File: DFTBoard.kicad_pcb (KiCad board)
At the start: 8 copper layers, 148.5 x 62 mm, 86 parts, among them CON1 AVR-JTAG-10, CON2 AVR-JTAG-10, J1 AUDIO JACK, J2 JACK_TRS_4PINS, J3 AUDIO JACK, J4 AUDIO JACK, J5 Micro_SD_Card_Det, J6 USB_A, J7 USB_B, SW1 TL6215RF200BDT, U10 VL53L0X, U11 APDS-9960, U12 MT41K256M16HA-125_E, U13 MT41K256M16HA-125_E, U5 xc7z020clg400, U6 TLV320AIC3104, U9 MIC2025-1YMM, Y1 Crystal, Y2 Crystal

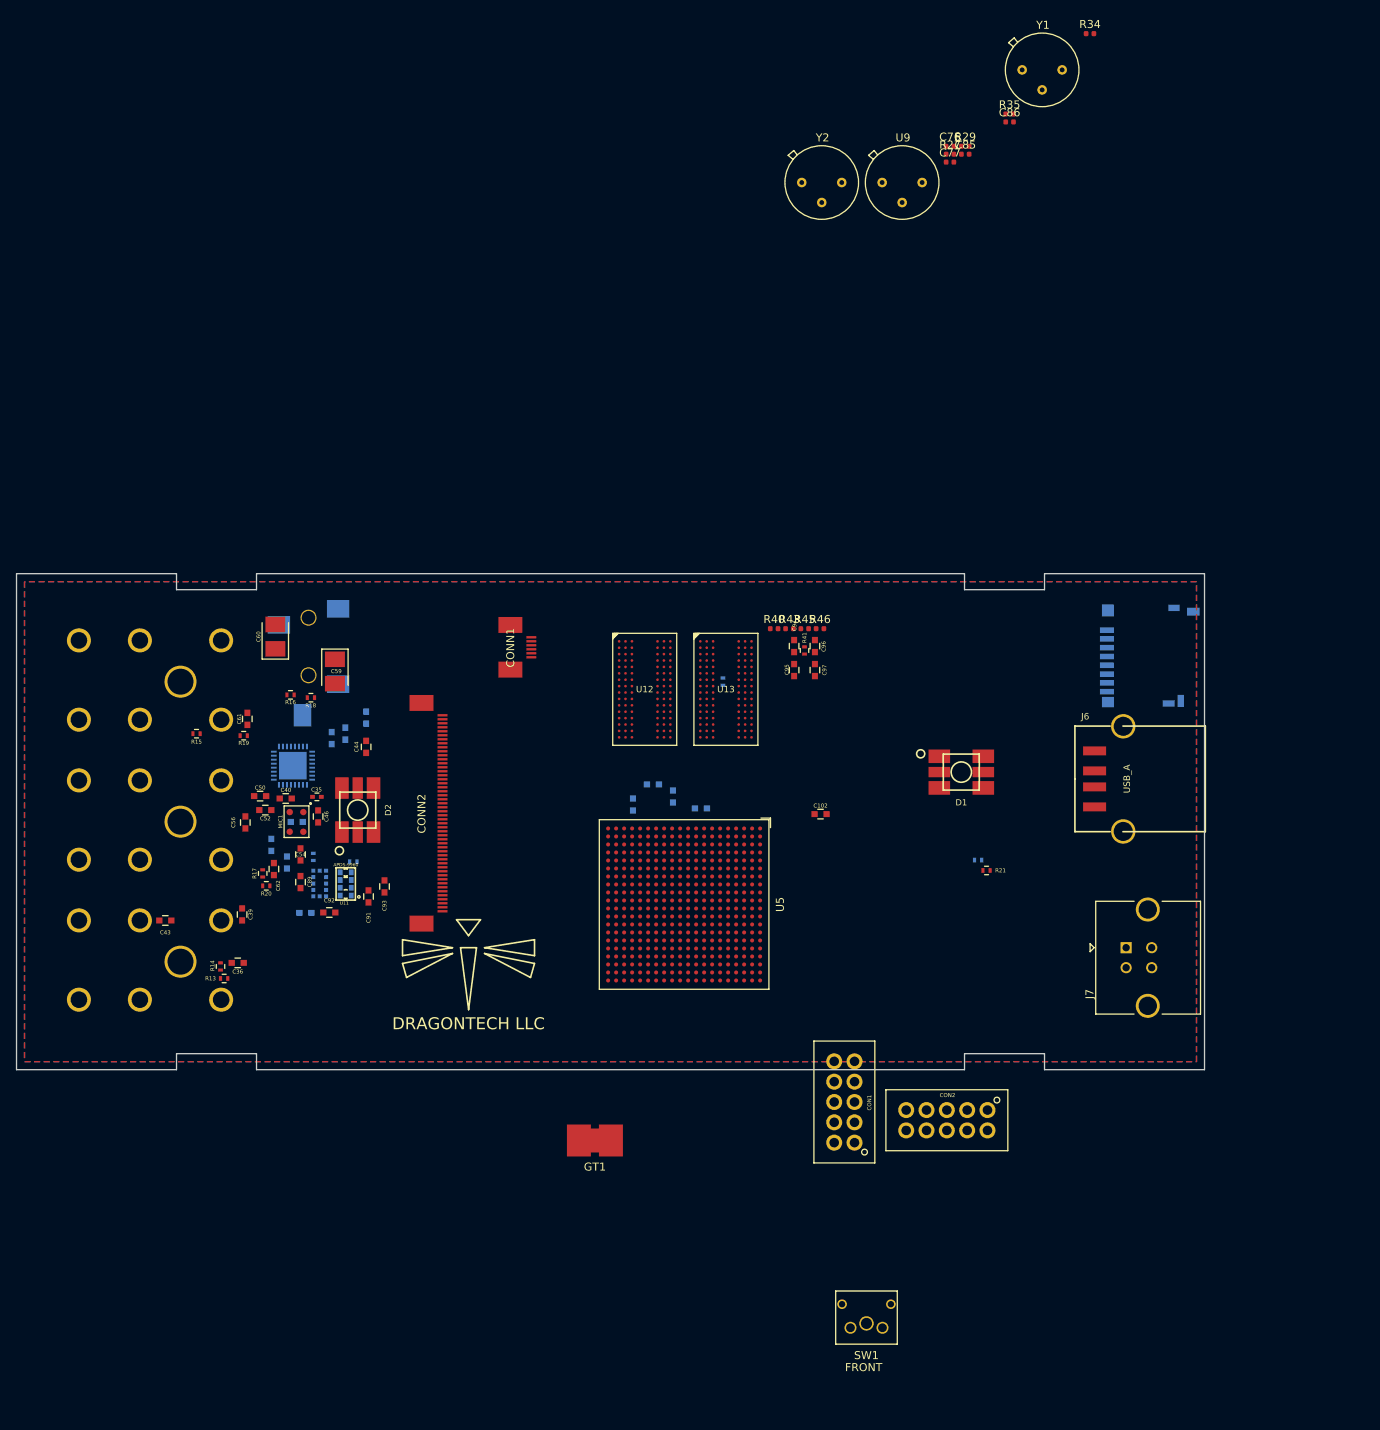
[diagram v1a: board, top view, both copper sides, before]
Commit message: random updates
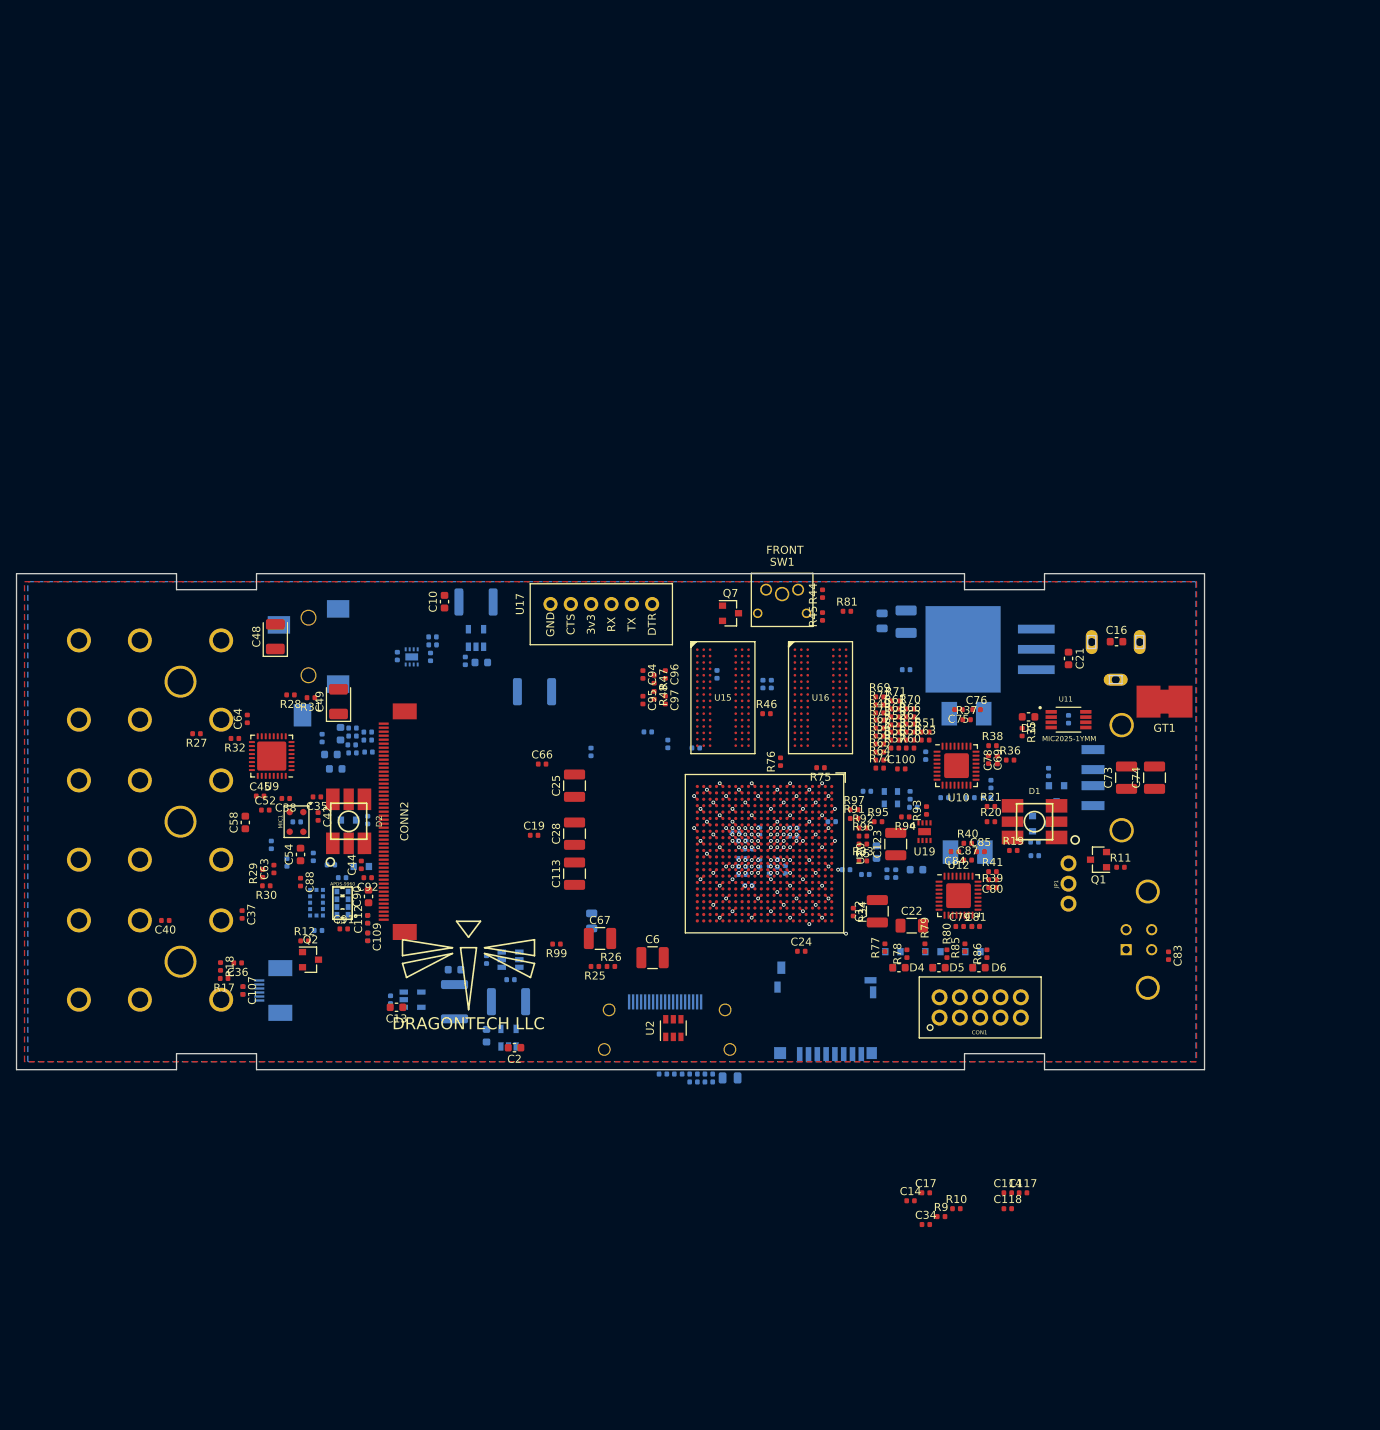
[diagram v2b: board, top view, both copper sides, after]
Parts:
- removed CON2: AVR-JTAG-10, DFTcustom:XilinxJTAG
- removed the J5 at (247.8, 103.2)
- removed the R37 at (143.6, 128.4)
- removed the R40 at (201.2, 99.9)
- removed the R41 at (205.0, 102.6)
- removed the U13 at (195.2, 107.5)
- added C1: .47uF, Capacitor_SMD:C_0402_1005Metric, B.Cu at (165.2, 141.2)
- added C10: 10uF, Capacitor_SMD:C_0603_1608Metric, F.Cu at (160.0, 96.5)
- added C100: 4.7uF, Capacitor_SMD:C_0402_1005Metric, F.Cu at (217.1, 117.4)
- added C101: .47uF, Capacitor_SMD:C_0402_1005Metric, B.Cu at (185.4, 112.8)
- added C103: .47uF, Capacitor_SMD:C_0402_1005Metric, B.Cu at (191.4, 114.8)
- added C108: 4.7uF, Capacitor_SMD:C_0402_1005Metric, B.Cu at (134.8, 145.1)
- added C109: .1uF, Capacitor_SMD:C_0402_1005Metric, F.Cu at (150.4, 138.4)
- added C11: 10uF, Capacitor_SMD:C_0603_1608Metric, B.Cu at (165.2, 150.8)
- added C110: 4.7uF, Capacitor_SMD:C_0402_1005Metric, B.Cu at (150.4, 138.4)
- added C111: .1uF, Capacitor_SMD:C_0402_1005Metric, B.Cu at (150.4, 136.2)
- added C112: 4.7uF, Capacitor_SMD:C_0402_1005Metric, F.Cu at (150.4, 136.2)
- added C113: 47uF, Capacitor_SMD:C_1210_3225Metric, F.Cu at (176.2, 130.5)
- added C114: 4.7uF, Capacitor_SMD:C_0402_1005Metric, F.Cu at (230.4, 170.4)
- added C115: 4.7uF, Capacitor_SMD:C_0402_1005Metric, B.Cu at (216.4, 130.5)
- added C116: .47uF, Capacitor_SMD:C_0402_1005Metric, B.Cu at (198.0, 127.4)
- added C117: .47uF, Capacitor_SMD:C_0402_1005Metric, F.Cu at (232.3, 170.4)
- added C118: .47uF, Capacitor_SMD:C_0402_1005Metric, F.Cu at (230.4, 172.4)
- added C119: .47uF, Capacitor_SMD:C_0402_1005Metric, B.Cu at (199.4, 125.2)
- added C12: 100uF, Capacitor_SMD:C_1210_3225Metric, F.Cu at (214.1, 135.2)
- added C120: .01uF, Capacitor_SMD:C_0402_1005Metric, B.Cu at (218.2, 120.7)
- added C121: .47uF, Capacitor_SMD:C_0402_1005Metric, B.Cu at (210.2, 130.0)
- added C122: 4.7uF, Capacitor_SMD:C_0402_1005Metric, B.Cu at (208.4, 124.0)
- added C123: 100uF, Capacitor_SMD:C_1210_3225Metric, F.Cu at (216.4, 126.8)
- added C13: 10uF, Capacitor_SMD:C_0603_1608Metric, F.Cu at (154.0, 147.2)
- added C14: .47uF, Capacitor_SMD:C_0402_1005Metric, F.Cu at (218.3, 171.4)
- added C15: .47uF, Capacitor_SMD:C_0402_1005Metric, B.Cu at (202.6, 130.0)
- added C16: 10uF, Capacitor_SMD:C_0603_1608Metric, F.Cu at (244.0, 101.5)
- added C17: .47uF, Capacitor_SMD:C_0402_1005Metric, F.Cu at (220.2, 170.4)
- added C18: .47uF, Capacitor_SMD:C_0402_1005Metric, B.Cu at (197.2, 129.6)
- added C19: 4.7uF, Capacitor_SMD:C_0402_1005Metric, F.Cu at (171.2, 125.7)
- added C2: 10uF, Capacitor_SMD:C_0603_1608Metric, F.Cu at (168.8, 152.2)
- added C20: 4.7uF, Capacitor_SMD:C_0402_1005Metric, B.Cu at (201.6, 129.2)
- added C21: 10uF, Capacitor_SMD:C_0603_1608Metric, F.Cu at (238.0, 103.6)
- added C22: 330uF, Capacitor_SMD:C_1206_3216Metric, F.Cu at (218.4, 137.0)
- added C23: .47uF, Capacitor_SMD:C_0402_1005Metric, B.Cu at (197.2, 126.4)
- added C24: 4.7uF, Capacitor_SMD:C_0402_1005Metric, F.Cu at (204.6, 140.2)
- added C25: 100uF, Capacitor_SMD:C_1210_3225Metric, F.Cu at (176.2, 119.5)
- added C26: 10uF, Capacitor_SMD:C_0603_1608Metric, B.Cu at (161.2, 142.5)
- added C27: 4.7uF, Capacitor_SMD:C_0402_1005Metric, B.Cu at (215.3, 130.5)
- added C28: 100uF, Capacitor_SMD:C_1210_3225Metric, F.Cu at (176.2, 125.5)
- added C29: .47uF, Capacitor_SMD:C_0402_1005Metric, B.Cu at (203.6, 125.8)
- added C3: 10uF, Capacitor_SMD:C_0603_1608Metric, B.Cu at (164.6, 104.1)
- added C30: .47uF, Capacitor_SMD:C_0402_1005Metric, B.Cu at (203.6, 124.8)
- added C31: .47uF, Capacitor_SMD:C_0402_1005Metric, B.Cu at (197.2, 130.6)
- added C32: 47uF, Capacitor_SMD:C_0805_2012Metric, B.Cu at (178.4, 136.4)
- added C33: 10uF, Capacitor_SMD:C_0603_1608Metric, B.Cu at (214.0, 127.8)
- added C34: .47uF, Capacitor_SMD:C_0402_1005Metric, F.Cu at (220.2, 174.4)
- added C37: 1uF, Capacitor_SMD:C_0402_1005Metric, F.Cu at (134.7, 135.6)
- added C38: 1uF, Capacitor_SMD:C_0402_1005Metric, F.Cu at (140.2, 121.1)
- added C4: .47uF, Capacitor_SMD:C_0402_1005Metric, B.Cu at (196.4, 125.4)
- added C42: 4.7uF, Capacitor_SMD:C_0402_1005Metric, F.Cu at (144.2, 123.3)
- added C45: 1uF, Capacitor_SMD:C_0402_1005Metric, F.Cu at (136.9, 120.8)
- added C47: .47uF, Capacitor_SMD:C_0402_1005Metric, B.Cu at (191.1, 155.5)
- added C48: 220uF Tant., Capacitor_Tantalum_SMD:CP_EIA-3528-12_Kemet-T, F.Cu at (138.8, 100.9)
- added C49: 220uF Tant., Capacitor_Tantalum_SMD:CP_EIA-3528-12_Kemet-T, F.Cu at (146.8, 109.0)
- added C5: 4.7uF, Capacitor_SMD:C_0402_1005Metric, B.Cu at (197.2, 128.6)
- added C6: 100uF, Capacitor_SMD:C_1210_3225Metric, F.Cu at (186.0, 141.0)
- added C63: .1uF, Capacitor_SMD:C_0402_1005Metric, F.Cu at (138.7, 129.9)
- added C64: .1uF, Capacitor_SMD:C_0402_1005Metric, F.Cu at (135.3, 111.2)
- added C65: .47uF, Capacitor_SMD:C_0402_1005Metric, B.Cu at (198.0, 132.0)
- added C66: 4.7uF, Capacitor_SMD:C_0402_1005Metric, F.Cu at (172.2, 116.8)
- added C67: 100uF, Capacitor_SMD:C_1210_3225Metric, F.Cu at (179.4, 138.6)
- added C68: .1uF, Capacitor_SMD:C_0402_1005Metric, B.Cu at (225.8, 121.0)
- added C69: 2.2uF, Capacitor_SMD:C_0402_1005Metric, F.Cu at (228.0, 116.2)
- added C7: 47uF, Capacitor_SMD:C_0805_2012Metric, B.Cu at (214.7, 98.9)
- added C70: .1uF, Capacitor_SMD:C_0402_1005Metric, B.Cu at (220.2, 115.8)
- added C71: .1uF, Capacitor_SMD:C_0402_1005Metric, B.Cu at (222.5, 121.0)
- added C72: .1uF, Capacitor_SMD:C_0402_1005Metric, B.Cu at (238.0, 111.2)
- added C73: 100uF, Capacitor_SMD:C_1210_3225Metric, F.Cu at (245.2, 118.5)
- added C74: 100uF, Capacitor_SMD:C_1210_3225Metric, F.Cu at (248.8, 118.5)
- added C77: .1uF, Capacitor_SMD:C_0402_1005Metric, B.Cu at (227.8, 121.0)
- added C78: .47uF, Capacitor_SMD:C_0402_1005Metric, F.Cu at (229.1, 116.3)
- added C79: .1uF, Capacitor_SMD:C_0402_1005Metric, F.Cu at (224.4, 137.1)
- added C8: .47uF, Capacitor_SMD:C_0402_1005Metric, B.Cu at (199.4, 129.2)
- added C80: 2.2uF, Capacitor_SMD:C_0402_1005Metric, F.Cu at (228.5, 131.2)
- added C81: .1uF, Capacitor_SMD:C_0402_1005Metric, F.Cu at (226.4, 137.1)
- added C82: .1uF, Capacitor_SMD:C_0402_1005Metric, B.Cu at (226.4, 137.1)
- added C83: 4.7uF, Capacitor_SMD:C_0402_1005Metric, F.Cu at (250.5, 140.8)
- added C86: .1uF, Capacitor_SMD:C_0402_1005Metric, B.Cu at (228.3, 119.3)
- added C87: .47uF, Capacitor_SMD:C_0402_1005Metric, F.Cu at (225.4, 128.8)
- added C88: .1uF, Capacitor_SMD:C_0402_1005Metric, F.Cu at (142.0, 131.6)
- added C9: 4.7uF, Capacitor_SMD:C_0402_1005Metric, B.Cu at (200.6, 130.0)
- added C98: .01uF, Capacitor_SMD:C_0402_1005Metric, B.Cu at (217.7, 105.0)
- added C99: 100uF, Capacitor_SMD:C_1210_3225Metric, B.Cu at (217.7, 99.0)
- added D3: BLUE LED, Capacitor_SMD:C_0603_1608Metric, F.Cu at (233.0, 110.9)
- added D4: BLUE LED, Capacitor_SMD:C_0603_1608Metric, F.Cu at (216.8, 142.2)
- added D5: BLUE LED, Capacitor_SMD:C_0603_1608Metric, F.Cu at (221.8, 142.2)
- added D6: BLUE LED, Capacitor_SMD:C_0603_1608Metric, F.Cu at (226.8, 142.2)
- added FB1: 120Ω @ 100 MHz, size 0603, Capacitor_SMD:C_0603_1608Metric, B.Cu at (219.0, 130.0)
- added J1: PJ-102A, PJ-102A:CUI_PJ-102A, B.Cu at (247.4, 101.5)
- added J8: Micro_SD_Card_Det, DFTcustom:AMPHENOL-114-00841-68, B.Cu at (207.6, 148.0)
- added J9: HDMI_A, DFTcustom:10029449-111RLF, B.Cu at (187.8, 152.5)
- added JP1: Jumper_3_Open, DFTcustom:JUMPER_3PIN, F.Cu at (238.0, 131.8)
- added L1: 2.2uH, Capacitor_SMD:C_1812_4532Metric, B.Cu at (171.2, 107.8)
- added L2: 2.2uH, Capacitor_SMD:C_1812_4532Metric, B.Cu at (163.9, 96.5)
- added L3: 2.2uH, Capacitor_SMD:C_1812_4532Metric, B.Cu at (168.0, 146.5)
- added L4: 2.2uH, Capacitor_SMD:C_1812_4532Metric, B.Cu at (161.2, 146.5)
- added Q1: IRLML2502, Package_TO_SOT_SMD:SOT-23, F.Cu at (241.8, 128.8)
- added Q10: IRLML2502, Package_TO_SOT_SMD:SOT-23, B.Cu at (226.1, 141.2)
- added Q2: IRLML2502, Package_TO_SOT_SMD:SOT-23, F.Cu at (143.2, 141.2)
- added Q3: IRLML2502, Package_TO_SOT_SMD:SOT-23, B.Cu at (234.5, 124.2)
- added Q4: IRLML2502, Package_TO_SOT_SMD:SOT-23, B.Cu at (148.0, 124.8)
- added Q5: IRLML2502, Package_TO_SOT_SMD:SOT-23, B.Cu at (236.5, 120.5)
- added Q6: IRLML2502, Package_TO_SOT_SMD:SOT-23, B.Cu at (149.6, 128.6)
- added Q7: IRLML2502, Package_TO_SOT_SMD:SOT-23, F.Cu at (195.8, 98.0)
- added Q8: IRLML2502, Package_TO_SOT_SMD:SOT-23, B.Cu at (216.1, 141.2)
- added Q9: IRLML2502, Package_TO_SOT_SMD:SOT-23, B.Cu at (221.1, 141.2)
- added R1: 100k, Resistor_SMD:R_0402_1005Metric, B.Cu at (168.2, 143.8)
- added R10: 4.7k, Resistor_SMD:R_0402_1005Metric, F.Cu at (224.0, 172.4)
- added R100: 24.9 1%, Resistor_SMD:R_0402_1005Metric, B.Cu at (212.8, 120.2)
- added R11: 100, Resistor_SMD:R_0402_1005Metric, F.Cu at (244.5, 129.7)
- added R12: 100, Resistor_SMD:R_0402_1005Metric, F.Cu at (142.5, 138.9)
- added R2: 100k, Resistor_SMD:R_0402_1005Metric, B.Cu at (153.2, 146.2)
- added R23: 100, Resistor_SMD:R_0402_1005Metric, B.Cu at (148.0, 121.5)
- added R24: 150, Resistor_SMD:R_0402_1005Metric, B.Cu at (150.0, 121.5)
- added R25: 4.7k, Resistor_SMD:R_0402_1005Metric, F.Cu at (178.8, 142.1)
- added R26: 4.7k, Resistor_SMD:R_0402_1005Metric, F.Cu at (180.8, 142.1)
- added R27: 100k, Resistor_SMD:R_0402_1005Metric, F.Cu at (129.0, 113.0)
- added R28: 100k, Resistor_SMD:R_0402_1005Metric, F.Cu at (140.8, 108.2)
- added R29: 100k, Resistor_SMD:R_0402_1005Metric, F.Cu at (137.3, 130.5)
- added R3: 100k, Resistor_SMD:R_0402_1005Metric, B.Cu at (162.6, 103.9)
- added R30: 49.9k, Resistor_SMD:R_0402_1005Metric, F.Cu at (137.7, 132.0)
- added R31: 49.9k, Resistor_SMD:R_0402_1005Metric, F.Cu at (143.3, 108.5)
- added R32: 49.9k, Resistor_SMD:R_0402_1005Metric, F.Cu at (133.8, 113.6)
- added R33: 10k, Resistor_SMD:R_0402_1005Metric, F.Cu at (212.3, 128.9)
- added R34: 47, Resistor_SMD:R_0402_1005Metric, F.Cu at (211.1, 135.3)
- added R35: 150, Resistor_SMD:R_0402_1005Metric, F.Cu at (232.2, 112.8)
- added R39: 10k, Resistor_SMD:R_0402_1005Metric, F.Cu at (228.5, 132.2)
- added R4: 100k, Resistor_SMD:R_0402_1005Metric, B.Cu at (154.1, 103.3)
- added R42: 10k, Resistor_SMD:R_0402_1005Metric, B.Cu at (145.8, 129.4)
- added R47: 10k 1%, Resistor_SMD:R_0402_1005Metric, F.Cu at (186.2, 106.2)
- added R48: 10k 1%, Resistor_SMD:R_0402_1005Metric, F.Cu at (186.2, 108.2)
- added R49: 240 1%, Resistor_SMD:R_0402_1005Metric, F.Cu at (214.4, 110.4)
- added R5: 100k, Resistor_SMD:R_0402_1005Metric, F.Cu at (212.3, 126.8)
- added R50: 100, Resistor_SMD:R_0402_1005Metric, B.Cu at (194.1, 105.6)
- added R51: 40.2 1%, Resistor_SMD:R_0402_1005Metric, F.Cu at (220.1, 112.8)
- added R52: 40.2 1%, Resistor_SMD:R_0402_1005Metric, F.Cu at (216.3, 111.9)
- added R53: 40.2 1%, Resistor_SMD:R_0402_1005Metric, F.Cu at (216.3, 112.8)
- added R54: 40.2 1%, Resistor_SMD:R_0402_1005Metric, F.Cu at (214.4, 113.3)
- added R55: 40.2 1%, Resistor_SMD:R_0402_1005Metric, F.Cu at (218.2, 112.8)
- added R56: 40.2 1%, Resistor_SMD:R_0402_1005Metric, F.Cu at (216.3, 113.8)
- added R57: 40.2 1%, Resistor_SMD:R_0402_1005Metric, F.Cu at (216.3, 114.8)
- added R58: 40.2 1%, Resistor_SMD:R_0402_1005Metric, F.Cu at (218.2, 113.8)
- added R59: 40.2 1%, Resistor_SMD:R_0402_1005Metric, F.Cu at (214.4, 114.3)
- added R6: 10k, Resistor_SMD:R_0402_1005Metric, B.Cu at (158.2, 103.4)
- added R60: 40.2 1%, Resistor_SMD:R_0402_1005Metric, F.Cu at (218.2, 114.8)
- added R61: 40.2 1%, Resistor_SMD:R_0402_1005Metric, F.Cu at (216.3, 109.9)
- added R62: 40.2 1%, Resistor_SMD:R_0402_1005Metric, F.Cu at (218.2, 111.8)
- added R63: 40.2 1%, Resistor_SMD:R_0402_1005Metric, F.Cu at (220.1, 113.8)
- added R64: 40.2 1%, Resistor_SMD:R_0402_1005Metric, F.Cu at (214.4, 116.3)
- added R65: 40.2 1%, Resistor_SMD:R_0402_1005Metric, F.Cu at (214.4, 115.3)
- added R66: 40.2 1%, Resistor_SMD:R_0402_1005Metric, F.Cu at (218.2, 110.9)
- added R67: 40.2 1%, Resistor_SMD:R_0402_1005Metric, F.Cu at (214.4, 112.3)
- added R68: 40.2 1%, Resistor_SMD:R_0402_1005Metric, F.Cu at (216.3, 110.9)
- added R69: 40.2 1%, Resistor_SMD:R_0402_1005Metric, F.Cu at (214.4, 108.4)
- added R7: 240 1%, Resistor_SMD:R_0402_1005Metric, B.Cu at (158.5, 101.9)
- added R70: 40.2 1%, Resistor_SMD:R_0402_1005Metric, F.Cu at (218.2, 109.9)
- added R71: 40.2 1%, Resistor_SMD:R_0402_1005Metric, F.Cu at (216.4, 108.9)
- added R72: 40.2 1%, Resistor_SMD:R_0402_1005Metric, F.Cu at (214.4, 109.4)
- added R73: 40.2 1%, Resistor_SMD:R_0402_1005Metric, F.Cu at (214.4, 111.3)
- added R74: 4.7k, Resistor_SMD:R_0402_1005Metric, F.Cu at (214.4, 117.3)
- added R75: 80.6, Resistor_SMD:R_0402_1005Metric, F.Cu at (207.0, 117.2)
- added R76: 80.6, Resistor_SMD:R_0402_1005Metric, F.Cu at (202.0, 116.5)
- added R77: 1k, Resistor_SMD:R_0402_1005Metric, F.Cu at (215.1, 139.8)
- added R78: 150, Resistor_SMD:R_0402_1005Metric, F.Cu at (217.8, 140.5)
- added R79: 1k, Resistor_SMD:R_0402_1005Metric, F.Cu at (220.1, 139.8)
- added R8: 4.7k, Resistor_SMD:R_0402_1005Metric, B.Cu at (158.5, 100.9)
- added R80: 150, Resistor_SMD:R_0402_1005Metric, F.Cu at (222.8, 140.5)
- added R81: 10k, Resistor_SMD:R_0402_1005Metric, F.Cu at (210.3, 97.7)
- added R82: 10k, Resistor_SMD:R_0402_1005Metric, B.Cu at (150.5, 115.3)
- added R83: 10k, Resistor_SMD:R_0402_1005Metric, B.Cu at (148.5, 115.4)
- added R84: 10k, Resistor_SMD:R_0402_1005Metric, B.Cu at (148.4, 114.4)
- added R85: 1k, Resistor_SMD:R_0402_1005Metric, F.Cu at (225.1, 139.8)
- added R86: 150, Resistor_SMD:R_0402_1005Metric, F.Cu at (227.8, 140.5)
- added R87: 33, Resistor_SMD:R_0402_1005Metric, B.Cu at (150.4, 113.8)
- added R88: 33, Resistor_SMD:R_0402_1005Metric, B.Cu at (148.5, 113.3)
- added R89: 33, Resistor_SMD:R_0402_1005Metric, B.Cu at (150.4, 112.8)
- added R9: 4.7k, Resistor_SMD:R_0402_1005Metric, F.Cu at (222.1, 173.4)
- added R90: 33, Resistor_SMD:R_0402_1005Metric, B.Cu at (148.5, 112.3)
- added R91: 20k, Resistor_SMD:R_0402_1005Metric, F.Cu at (211.2, 123.6)
- added R92: 20k, Resistor_SMD:R_0402_1005Metric, F.Cu at (212.3, 124.8)
- added R93: 20k, Resistor_SMD:R_0402_1005Metric, F.Cu at (220.2, 122.6)
- added R94: 20k, Resistor_SMD:R_0402_1005Metric, F.Cu at (217.6, 123.4)
- added R95: 20k, Resistor_SMD:R_0402_1005Metric, F.Cu at (214.2, 124.0)
- added R96: 20k, Resistor_SMD:R_0402_1005Metric, F.Cu at (212.3, 125.8)
- added R97: 20k, Resistor_SMD:R_0402_1005Metric, F.Cu at (211.2, 122.5)
- added R98: 4.7k, Resistor_SMD:R_0402_1005Metric, B.Cu at (218.6, 122.2)
- added R99: 47k, Resistor_SMD:R_0402_1005Metric, F.Cu at (174.0, 139.3)
- added U1: LM3880, Package_TO_SOT_SMD:SOT-23-6, B.Cu at (168.2, 141.2)
- added U10: USB3320, Package_DFN_QFN:QFN-32-1EP_5x5mm_P0.5mm_EP3.1x3.1mm, F.Cu at (224.0, 117.0)
- added U11: MIC2025-1YMM, SOP65P490X110-8N:SOP65P490X110-8N, F.Cu at (238.0, 111.2)
- added U12: USB3320, Package_DFN_QFN:QFN-32-1EP_5x5mm_P0.5mm_EP3.1x3.1mm, F.Cu at (224.2, 133.2)
- added U16: MT41K256M16HA-125_E, DFTcustom:FBGA-96-DDR3-SDRAM, F.Cu at (207.0, 108.5)
- added U17: FTDITypeUART, DFTcustom:FTDI_CONN, F.Cu at (179.6, 96.8)
- added U18: ABRACON-ASDMB, XTAL_ASDMB-24.000MHZ-LC-T:XTAL_ASDMB-24.000MHZ-LC-T, B.Cu at (215.8, 121.0)
- added U19: S25FL256SAGNFI001, DFTcustom:WSON-8, F.Cu at (220.0, 125.2)
- added U2: LM3880, Package_TO_SOT_SMD:SOT-23-6, F.Cu at (188.6, 149.8)
- added U20: xc7z020clg484, DFTcustom:BGA-484_19.0x19.0mm_Layout22x22_P0.80mm_dia0.40mm, F.Cu at (200.0, 128.0)
- added U3: SC189 - 1.0V, Package_TO_SOT_SMD:SOT-23-5, B.Cu at (168.0, 151.0)
- added U4: SC189 - 3.3V, Package_TO_SOT_SMD:SOT-23-5, B.Cu at (163.9, 101.0)
- added U7: SC189 - 1.8V, Package_TO_SOT_SMD:SOT-23-5, B.Cu at (156.0, 146.2)
- C102, C46: value 4.7uF -> .47uF; footprint Capacitors_SMD:C_0603 -> Capacitor_SMD:C_0402_1005Metric; moved to B.Cu
- C104, C36, C40, C52, C53, C92, C94, C95, C96, C97: footprint Capacitors_SMD:C_0603 -> Capacitor_SMD:C_0402_1005Metric
- C105, C106: value .47uF -> .01uF; footprint Capacitors_SMD:C_0603 -> Capacitor_SMD:C_0402_1005Metric
- C107: value .47uF -> .1uF; footprint Capacitors_SMD:C_0603 -> Capacitor_SMD:C_0402_1005Metric; moved to F.Cu
- C35: footprint Capacitors_SMD:C_0402 -> Capacitor_SMD:C_0402_1005Metric
- C39: value 1uF -> .1uF; footprint Capacitors_SMD:C_0603 -> Capacitor_SMD:C_0402_1005Metric; moved to B.Cu
- C41: value .1uF -> 10uF; footprint Capacitors_SMD:C_0603 -> Capacitor_SMD:C_0603_1608Metric
- C43, C62: footprint Capacitors_SMD:C_0603 -> Capacitor_SMD:C_0402_1005Metric; moved to B.Cu
- C44, C91: value 10uF -> 1uF; footprint Capacitors_SMD:C_0603 -> Capacitor_SMD:C_0402_1005Metric
- C50: value 1uF -> .47uF; footprint Capacitors_SMD:C_0603 -> Capacitor_SMD:C_0402_1005Metric; moved to B.Cu
- C51, C54: footprint Capacitors_SMD:C_0603 -> Capacitor_SMD:C_0603_1608Metric
- C55: value .1uF -> .47uF; footprint Capacitors_SMD:C_0603 -> Capacitor_SMD:C_0402_1005Metric
- C56: value 10uF -> .1uF; footprint Capacitors_SMD:C_0603 -> Capacitor_SMD:C_0402_1005Metric; moved to B.Cu
- C57: value 10uF -> 4.7uF; footprint Capacitors_SMD:C_0603 -> Capacitor_SMD:C_0402_1005Metric
- C58: value .1uF -> 10uF; footprint Capacitors_SMD:C_0603 -> Capacitor_SMD:C_0603_1608Metric; moved to F.Cu
- C59: value 220uF Tant. -> 4.7uF; footprint Capacitors_Tantalum_SMD:CP_Tantalum_Case-T_EIA-3528-12_Reflow -> Capacitor_SMD:C_0402_1005Metric; moved to B.Cu
- C60: value 220uF Tant. -> 10uF; footprint Capacitors_Tantalum_SMD:CP_Tantalum_Case-T_EIA-3528-12_Reflow -> Capacitor_SMD:C_0603_1608Metric; moved to B.Cu
- C61: value .1uF -> 47uF; footprint Capacitors_SMD:C_0603 -> Capacitor_SMD:C_0805_2012Metric; moved to B.Cu
- C89: value .1uF -> 4.7uF; footprint Capacitors_SMD:C_0603 -> Capacitor_SMD:C_0402_1005Metric; moved to B.Cu
- C90: value 4.7uF -> 10uF; footprint Capacitors_SMD:C_0603 -> Capacitor_SMD:C_0603_1608Metric; moved to F.Cu
- C93: value 1uF -> .01uF; footprint Capacitors_SMD:C_0603 -> Capacitor_SMD:C_0402_1005Metric; moved to B.Cu
- CONN1, J6, J7: moved to B.Cu
- R13, R15, R16: value 100k -> 100; footprint Resistors_SMD:R_0402 -> Resistor_SMD:R_0402_1005Metric; moved to B.Cu
- R14: value 49.9k -> 100; footprint Resistors_SMD:R_0402 -> Resistor_SMD:R_0402_1005Metric; moved to B.Cu
- R17, R18: footprint Resistors_SMD:R_0402 -> Resistor_SMD:R_0402_1005Metric
- R19, R20: value 49.9k -> 100; footprint Resistors_SMD:R_0402 -> Resistor_SMD:R_0402_1005Metric
- R21: value 4.7k -> 150; footprint Resistors_SMD:R_0402 -> Resistor_SMD:R_0402_1005Metric
- R22: value 4.7k -> 100; footprint Resistors_SMD:R_0402 -> Resistor_SMD:R_0402_1005Metric
- R36: footprint Resistors_SMD:R_0402 -> Resistor_SMD:R_0402_1005Metric; moved to F.Cu
- R43: value 240 1% -> 10k; moved to B.Cu
- R44: value 100 -> 10k; footprint Resistors_SMD:R_0402 -> Resistor_SMD:R_0402_1005Metric; moved to F.Cu
- R45: value 80.6 -> 150
- R46: value 80.6 -> 240 1%
- U5: value xc7z020clg400 -> TLV62080DSGx; footprint Package_BGA:BGA-400_21.0x21.0mm_Layout20x20_P1.0mm -> Package_SON:WSON-8-1EP_2x2mm_P0.5mm_EP0.9x1.6mm; moved to B.Cu
- U6: value TLV320AIC3104 -> LM1085-5.0; footprint Housings_DFN_QFN:QFN-32-1EP_5x5mm_Pitch0.5mm -> Package_TO_SOT_SMD:TO-263-3_TabPin2
- U9: value MIC2025-1YMM -> TLV320AIC3104; footprint Crystal:Crystal_HC35-U -> Package_DFN_QFN:QFN-32-1EP_5x5mm_P0.5mm_EP3.65x3.65mm
- Y1, Y2: value Crystal -> ABM3-24.000MHZ-D2Y-T; footprint Crystal:Crystal_HC35-U -> ABM3-12.000MHZ-B2-T:XTAL500X320X130N; moved to B.Cu
- moved C43 109.0 mm to (233.8, 128.2), turned to 0 degrees
- moved R15 106.6 mm to (235.5, 117.8), turned to 90 degrees
- moved U9 104.7 mm to (138.4, 115.8), turned to 180 degrees
- moved R13 102.7 mm to (233.8, 126.5)
- moved R40 102.4 mm to (225.4, 126.7)
- moved R19 97.3 mm to (231.1, 127.6), turned to 0 degrees
- moved SW1 96.9 mm to (202.2, 93.0), turned to 180 degrees
- moved R41 94.7 mm to (228.5, 130.2)
- moved C85 91.3 mm to (227.0, 127.8)
- moved R20 90.9 mm to (228.3, 124.0), turned to 0 degrees
- moved GT1 89.9 mm to (250.0, 109.0)
- moved U6 88.4 mm to (228.2, 102.5)
- moved C84 87.2 mm to (223.8, 127.8), turned to 180 degrees
- moved Y2 86.2 mm to (225.4, 127.8)
- moved R36 83.1 mm to (230.7, 116.3), turned to 0 degrees
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- renumbered C76 to C75, C77 to C76, C85 to C84, C86 to C85, J1 to J2, J4 to J3, J3 to J4, J2 to J5, R27 to R37, R29 to R38, R34 to R40, R35 to R41, U10 to U13, U11 to U14, U12 to U15
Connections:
- C102 pad 1: Net-(C100-Pad1) -> +1V35
- C104 pad 1: Net-(C100-Pad1) -> +1V35
- C105 pad 1: Net-(C100-Pad1) -> /DDR3/VREF
- C106 pad 1: Net-(C100-Pad1) -> /DDR3/VREF
- C107 pad 1: Net-(C100-Pad1) -> +3V3
- C39 pad 1: /Audio/JACK_INC_P -> GND
- C39 pad 2: /Audio/JACK_IN_P -> +1V8
- C40 pad 1: /Audio/SIG_F -> /Audio/JACK_INC_N
- C40 pad 2: /Audio/SIGC_F -> /Audio/JACK_IN_N
- C41 pad 2: +1.8V -> +1V8
- C43 pad 1: /Audio/JACK_INC_N -> +5V
- C43 pad 2: /Audio/JACK_IN_N -> GND
- C44 pad 1: GND -> +5V
- C44 pad 2: +1.8V -> GND
- C46 pad 1: /Audio/MICBIAS -> +3V3
- C46 pad 2: GNDA -> GND
- C50 pad 1: GNDA -> +3V3
- C50 pad 2: Net-(C50-Pad2) -> GND
- C51 pad 1: +1.8V -> +1V8
- C53 pad 1: +1.8V -> +1V8
- C55 pad 1: GNDA -> +3V3
- C55 pad 2: +3V3 -> GND
- C57 pad 2: GNDA -> GND
- C58 pad 1: +3V3 -> GNDA
- C58 pad 2: GNDA -> +3V3
- C59 pad 1: /Audio/HPRCOM_N -> +3V3
- C59 pad 2: /Audio/HPRCOM_MC -> GND
- C60 pad 1: /Audio/HPRCOM_P -> +3V3
- C60 pad 2: /Audio/HPRCOM_PC -> GNDA
- C61 pad 1: JD_ROUT -> +3V3
- C62 pad 1: JD_LOUT -> +3V3
- C62 pad 2: GND -> GNDA
- C90 pad 1: +3V3 -> GND
- C90 pad 2: GND -> +3V3
- C93 pad 1: GND -> /DDR3/VREF
- C93 pad 2: +3V3 -> GND
- CON1 pad 4: +1.8V -> +1V8
- CONN1 pad 2: I2C_SDIN -> I2C33_SDA
- CONN1 pad 3: I2C_SCLK -> I2C33_SCLK
- CONN1 pad 4: (no net) -> TOUCH_RST#
- CONN1 pad 5: (no net) -> TOUCH_INT#
- CONN2 pad 2: (no net) -> Net-(CONN2-Pad2)
- CONN2 pad 3: (no net) -> Net-(CONN2-Pad3)
- CONN2 pad 4: (no net) -> Net-(CONN2-Pad4)
- CONN2 pad 40: +1.8V -> +1V8
- CONN2 pad 41: +1.8V -> +1V8
- CONN2 pad 5: (no net) -> Net-(CONN2-Pad5)
- D2 pad 1: /Audio/LED_1RC -> /Audio/LED_2RC
- D2 pad 2: /Audio/LED_1GC -> /Audio/LED_2GC
- D2 pad 3: /Audio/LED_1BC -> /Audio/LED_2BC
- D2 pad 4: /Audio/LED_1BA -> /Audio/LED_2BA
- D2 pad 5: /Audio/LED_1GA -> /Audio/LED_2GA
- D2 pad 6: /Audio/LED_1RA -> /Audio/LED_2RA
- J3 pad R: /Audio/LOUT_P -> LOUT_N
- J3 pad T: /Audio/LOUT_N -> LOUT_P
- J4 pad R: /Audio/ROUT_P -> ROUT_N
- J4 pad T: /Audio/ROUT_N -> ROUT_P
- J6 pad 1: (no net) -> USBH_VBUS
- J6 pad 2: (no net) -> USBH_D_N
- J6 pad 3: (no net) -> USBH_D_P
- J7 pad 1: (no net) -> USBD_VBUS
- J7 pad 2: (no net) -> USBD_D_N
- J7 pad 3: (no net) -> USBD_D_P
- R13 pad 1: +3V3 -> Net-(Q3-Pad1)
- R13 pad 2: /Audio/INSWITCH -> LED_1G_CTRL
- R14 pad 1: JD_IN -> Net-(Q4-Pad1)
- R14 pad 2: /Audio/INSWITCH -> LED_2G_CTRL
- R15 pad 1: /Audio/RSWITCH -> Net-(Q5-Pad1)
- R15 pad 2: +1.8V -> LED_1B_CTRL
- R16 pad 1: /Audio/HPSWITCH -> Net-(Q6-Pad1)
- R16 pad 2: +3V3 -> LED_2B_CTRL
- R17 pad 1: /Audio/LSWITCH -> +1V8
- R17 pad 2: +1.8V -> /Audio/INSWITCH
- R18 pad 1: (no net) -> JD_IN
- R18 pad 2: /Audio/HPSWITCH -> /Audio/INSWITCH
- R19 pad 1: JD_ROUT -> +5V
- R19 pad 2: /Audio/RSWITCH -> /Audio/LED_1RA
- R20 pad 1: JD_LOUT -> +5V
- R20 pad 2: /Audio/LSWITCH -> /Audio/LED_1GA
- R21 pad 1: I2C3v3_SCLK -> +5V
- R21 pad 2: +3V3 -> /Audio/LED_1BA
- R22 pad 1: I2C3v3_SDIN -> +5V
- R22 pad 2: +3V3 -> /Audio/LED_2RA
- R36 pad 1: +1.8V -> Net-(R36-Pad1)
- R36 pad 2: Net-(R36-Pad2) -> USBH_VBUS
- R38 pad 1: (no net) -> Net-(R38-Pad1)
- R41 pad 1: (no net) -> Net-(R41-Pad1)
- R43 pad 1: Net-(R43-Pad1) -> +1V8
- R43 pad 2: GND -> RF_IRQ
- R44 pad 1: DDR3_CK_P -> +1V8
- R44 pad 2: DDR3_CK_N -> TEMPO_SW
- R45 pad 1: Net-(R45-Pad1) -> +5V
- R45 pad 2: +1V35 -> /Sensors/TEMPO_LED_R
- SW1 pad 3: (no net) -> /Sensors/TEMPO_LED_D
- SW1 pad 4: (no net) -> /Sensors/TEMPO_LED_R
- U13 pad 10: (no net) -> I2C18_SCLK
- U13 pad 5: Net-(R36-Pad2) -> Net-(R42-Pad2)
- U13 pad 9: (no net) -> I2C18_SDIN
- U14 pad 1: (no net) -> I2C33_SDA
- U14 pad 7: (no net) -> I2C33_SCLK
- U15 pad L8: Net-(R40-Pad1) -> Net-(R46-Pad1)
- U6 pad 1: I2S_MCLK -> GND
- U6 pad 2: I2S_BCLK -> Net-(C21-Pad1)
- U6 pad 3: I2S_LRCLK -> Net-(C16-Pad1)
- U9 pad 1: (no net) -> I2S_MCLK
- U9 pad 2: (no net) -> I2S_BCLK
- U9 pad 3: GND -> I2S_LRCLK
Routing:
- net GND: track 0.00 -> 39.0 mm, vias 0 -> 68
- net +1V8: track 0.00 -> 11.3 mm, vias 0 -> 26
- net +1V0: track 0.00 -> 9.05 mm, vias 0 -> 15
- net +3V3: track 0.00 -> 5.09 mm, vias 0 -> 15
- net +1V35: track 0.00 -> 5.09 mm, vias 0 -> 9
- added copper zone on 1V8, net +1V8
- added copper zone on B.Cu, net +3V3
- added copper zone on F.Cu, net GND
- removed copper zone on Core_Supply_5V, net +1.0V
- removed copper zone on Core_Supply_5V, net +1.2V
- removed copper zone on B.Cu, net +1.8V
- removed copper zone on Core_Supply_5V, net +5V
- removed copper zone on GND0, net GND
- removed copper zone on GND1, net GND
- removed copper zone on SIGNAL1, net GND
- removed copper zone on SIGNAL2, net GND
- removed copper zone on SIGNAL3, net GND
- removed copper zone on F.Cu, net GNDA
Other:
- net class Analog removed
- net class Config removed
- net class Crystal removed
- net class DDR_Differential added: clearance 0.102, trace_width 0.13, via_dia 0.48, via_drill 0.25
- net class DDR_Single added: clearance 0.102, trace_width 0.13, via_dia 0.48, via_drill 0.25
- net class Default: via_dia 0.45 -> 0.48; via_drill 0.22 -> 0.25
- net class GPIF removed
- net class HDMI: via_dia 0.45 -> 0.48; via_drill 0.22 -> 0.25
- net class LEDs removed
- net class Peripherals removed
- net class Power: trace_width 0.39 -> 0.13; via_dia 0.7 -> 0.48; via_drill 0.4 -> 0.25
- net class UI removed
- net class USB SIG: via_dia 0.45 -> 0.48; via_drill 0.22 -> 0.25
